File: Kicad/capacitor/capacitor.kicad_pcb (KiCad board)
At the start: 2 copper layers, 100 x 35 mm, 142 parts, among them K1 Capacitor

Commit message: Update Capacitor
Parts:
- removed H12, H6, H9: KEYSTONE-9056, tronixio:KEYSTONE-9056
- added H1: KEYSTONE-9056, tronixio:KEYSTONE-9056, F.Cu at (103.0, 97.0)
- added H2: KEYSTONE-9056, tronixio:KEYSTONE-9056, F.Cu at (197.0, 97.0)
- added H4: KEYSTONE-9056, tronixio:KEYSTONE-9056, F.Cu at (103.0, 68.0)
- moved H3 98.4 mm to (197.0, 68.0)

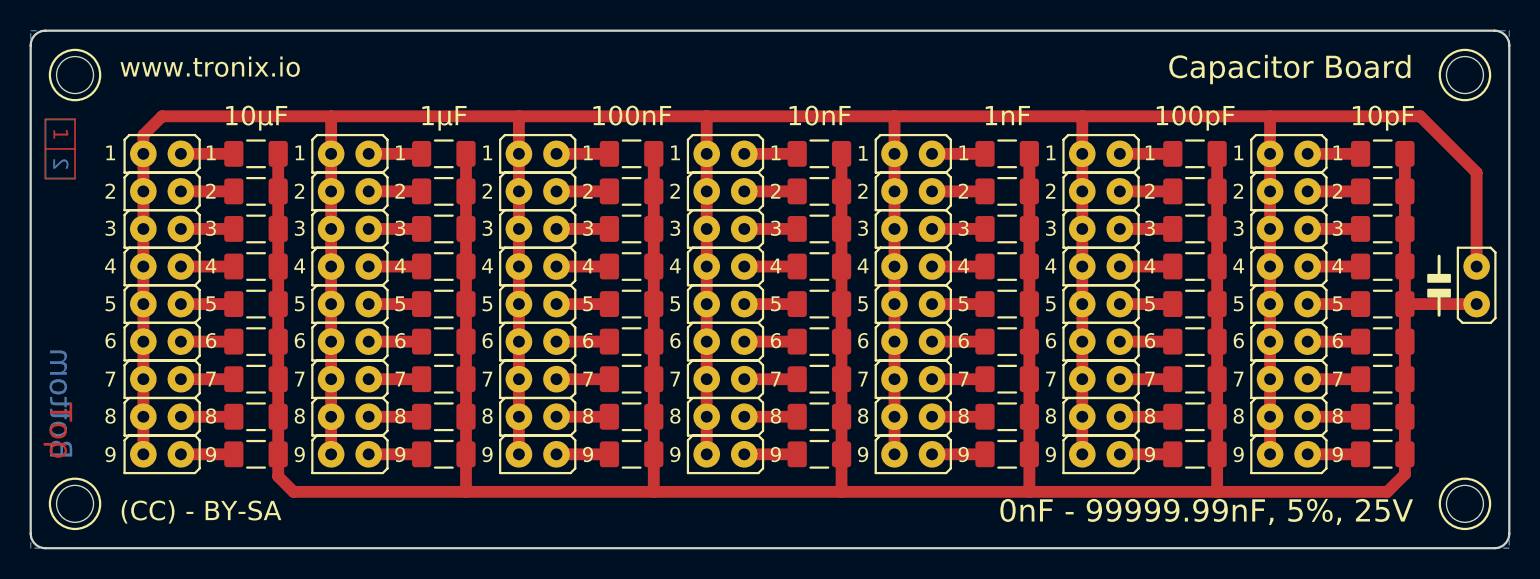
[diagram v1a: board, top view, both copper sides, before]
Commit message: Update
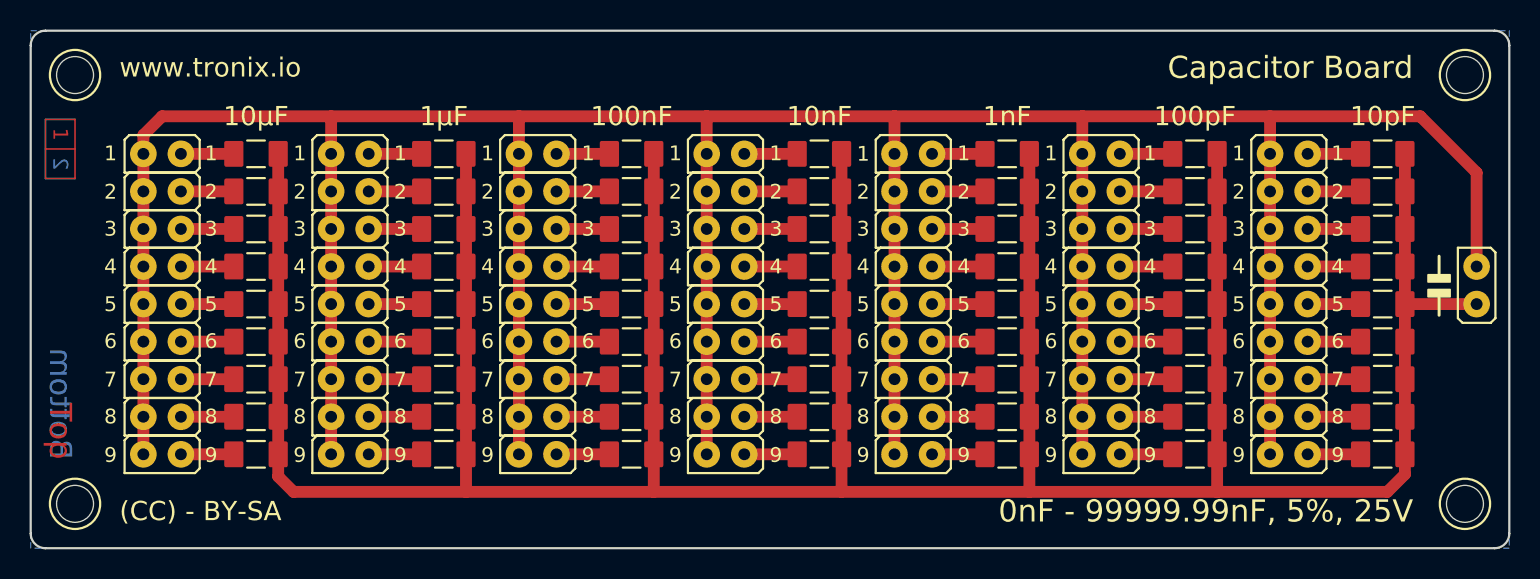
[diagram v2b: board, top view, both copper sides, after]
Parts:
- C1, C10, C11, C12, C13, C14, C15, C16, C17, C18, C19, C2, C20, C21, C22, C23, C24, C25, C26, C27, C28, C29, C3, C30, C31, C32, C33, C34, C35, C36, C37, C38, C39, C4, C40, C41, C42, C43, C44, C45, C46, C47, C48, C49, C5, C50, C51, C52, C53, C54, C55, C56, C57, C58, C59, C6, C60, C61, C62, C63, C7, C8, C9: footprint tronixio:CAPACITOR-1206 -> tronixio:CAPACITOR-SMD-1206
